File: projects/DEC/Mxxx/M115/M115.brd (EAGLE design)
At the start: 125.7 x 62.2 mm, 8 parts, among them IC1 7410N, IC2 7410N, IC3 7410N

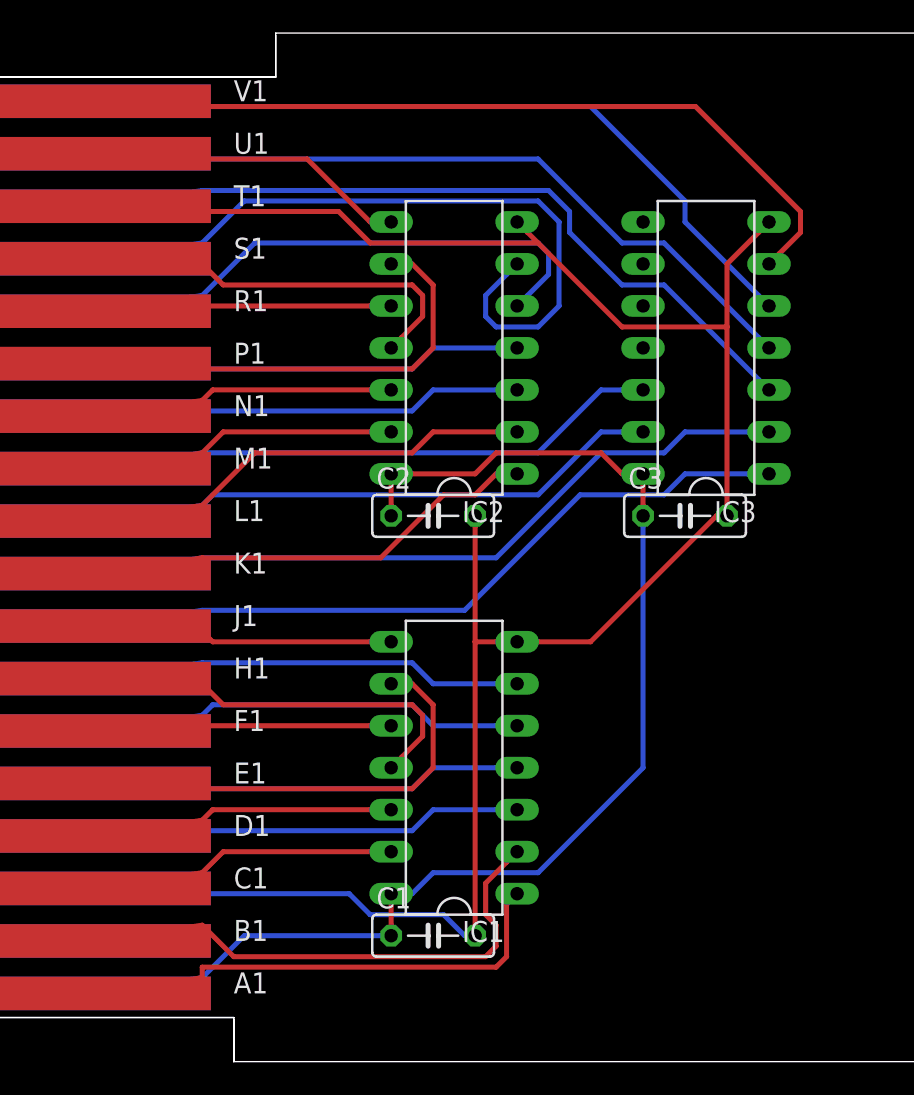
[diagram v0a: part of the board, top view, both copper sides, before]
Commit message: Walk the project tree, making things pass current design rules.
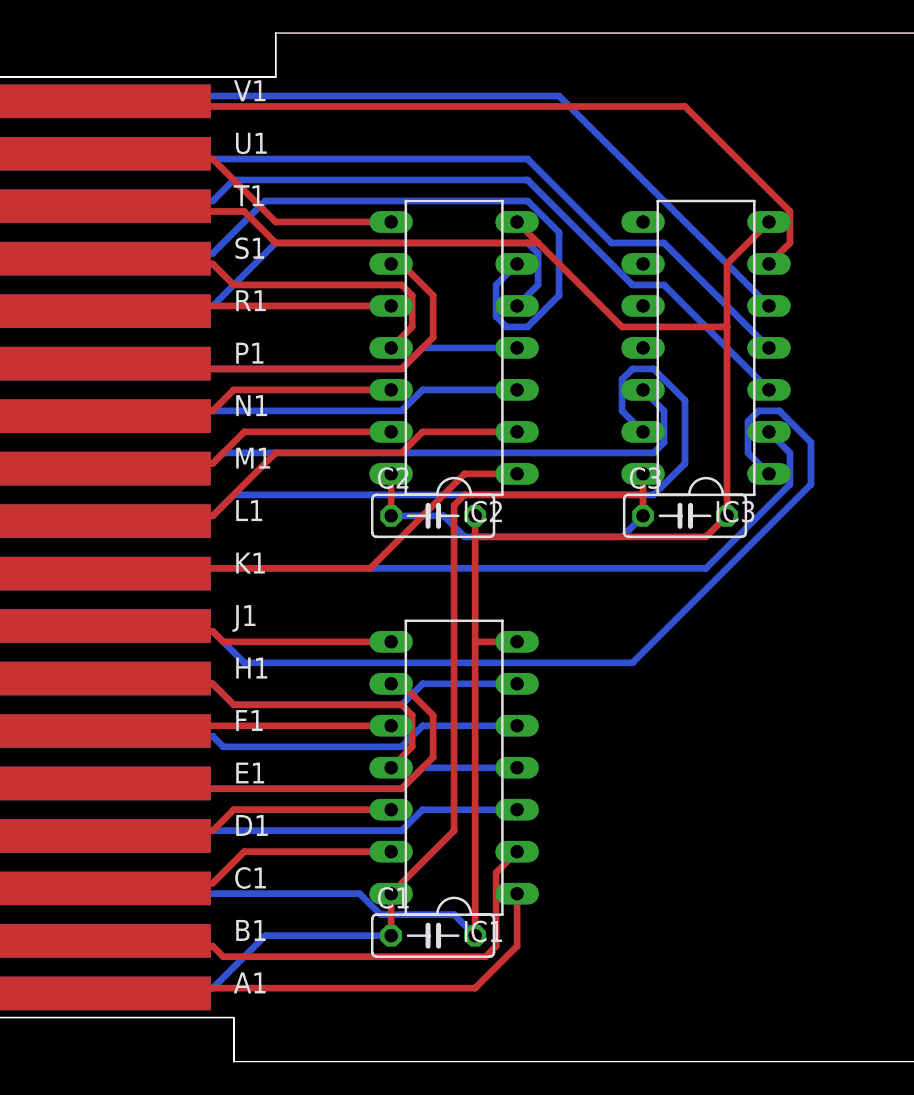
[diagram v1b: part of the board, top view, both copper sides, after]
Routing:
- net J2: track 43.8 -> 59.4 mm
- net L2: track 34.6 -> 49.1 mm
- net K2: track 43.6 -> 47.5 mm
- net M2: track 34.4 -> 38.3 mm
- net VCC: track 76.1 -> 79.6 mm
- net S2: track 43.6 -> 42.2 mm
- net B1: track 31.7 -> 30.7 mm
- net H1: track 24.1 -> 23.4 mm
- net V1: track 48.8 -> 48.1 mm
- net S1: track 24.1 -> 23.4 mm
- net P1: track 27.4 -> 26.8 mm
- net E1: track 27.4 -> 26.8 mm
- net H2: track 25.7 -> 26.3 mm
- net R2: track 32.6 -> 32.0 mm
